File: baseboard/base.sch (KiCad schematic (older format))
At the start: 35 parts, among them J1 Conn_02x05_Odd_Even, J2 Barrel_Jack, J3 Barrel_Jack, J4 Conn_01x03_Male, Q1 BSS138, Q2 BSS138, Q3 BSS138, Q4 BSS138, Q5 BSS138, SW1 SW_Push, SW2 SW_Push, SW3 SW_Push, SW4 SW_Push, SW5 SW_Push, SW6 SW_Push, U1 WeMos_mini, U2 DS3231RTCModule, U3 NCH6100HVNixiePSU, U4 LM2596BuckConverterModule

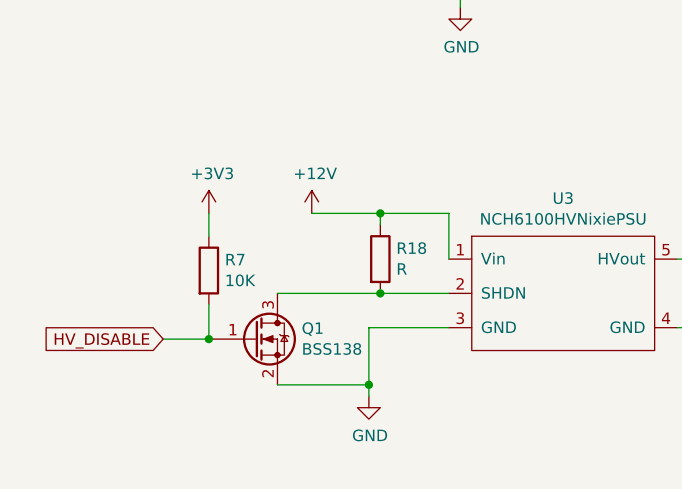
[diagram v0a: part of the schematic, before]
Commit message: Fix pulldown
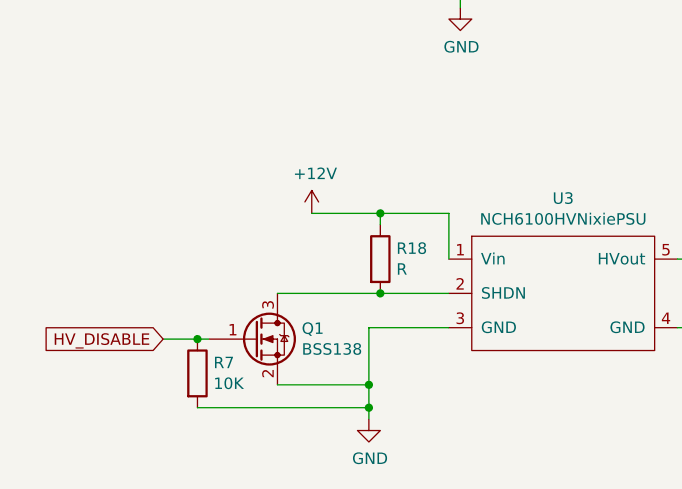
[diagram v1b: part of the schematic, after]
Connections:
- net +3V3: no longer R7.1
- net GND: now also R7.2
- net HV_DISABLE: now also R7.1; no longer R7.2
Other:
- moved on the sheet: R7
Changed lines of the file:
@@
 L power:GND #PWR0130
 U 1 1 5DC41A7F
-P 2050 6750
-F 0 "#PWR0130" H 2050 6500 50  0001 C CNN
-F 1 "GND" H 2055 6577 50  0000 C CNN
-F 2 "" H 2050 6750 50  0001 C CNN
-F 3 "" H 2050 6750 50  0001 C CNN
-	1    2050 6750
+P 2050 6850
+F 0 "#PWR0130" H 2050 6600 50  0001 C CNN
+F 1 "GND" H 2055 6677 50  0000 C CNN
+F 2 "" H 2050 6850 50  0001 C CNN
+F 3 "" H 2050 6850 50  0001 C CNN
+	1    2050 6850
 	1    0    0    -1
 $EndComp
@@
 	1650 6700 2050 6700
 Connection ~ 2050 6700
-Wire Wire Line
-	2050 6700 2050 6750
-Wire Wire Line
-	1150 6500 1350 6500
 $Comp
 L Transistor_FET:BSS138 Q5
@@
 Text GLabel 2550 1550 2    50   Input ~ 0
 SW_2
-$Comp
-L Device:R R7
-U 1 1 5DE5FC03
-P 1350 6200
-F 0 "R7" H 1420 6246 50  0000 L CNN
-F 1 "10K" H 1420 6155 50  0000 L CNN
-F 2 "Resistor_SMD:R_0805_2012Metric_Pad1.15x1.40mm_HandSolder" V 1280 6200 50  0001 C CNN
-F 3 "~" H 1350 6200 50  0001 C CNN
-	1    1350 6200
-	1    0    0    -1
-$EndComp
-$Comp
-L power:+3V3 #PWR0120
-U 1 1 5DE60E59
-P 1350 5950
-F 0 "#PWR0120" H 1350 5800 50  0001 C CNN
-F 1 "+3V3" H 1365 6123 50  0000 C CNN
-F 2 "" H 1350 5950 50  0001 C CNN
-F 3 "" H 1350 5950 50  0001 C CNN
-	1    1350 5950
-	1    0    0    -1
-$EndComp
+Wire Wire Line
+	2100 4700 3250 4700
+Wire Wire Line
+	2100 4550 3200 4550
 $Comp
 L Transistor_FET:BSS138 Q1
@@
 $EndComp
 Wire Wire Line
-	1350 6050 1350 5950
-Wire Wire Line
-	1350 6350 1350 6500
-Connection ~ 1350 6500
-Wire Wire Line
-	2100 4700 3250 4700
-Wire Wire Line
-	2100 4550 3200 4550
+	1150 6500 1300 6500
+$Comp
+L Device:R R7
+U 1 1 5DE5FC03
+P 1300 6650
+F 0 "R7" H 1370 6696 50  0000 L CNN
+F 1 "10K" H 1370 6605 50  0000 L CNN
+F 2 "Resistor_SMD:R_0805_2012Metric_Pad1.15x1.40mm_HandSolder" V 1230 6650 50  0001 C CNN
+F 3 "~" H 1300 6650 50  0001 C CNN
+	1    1300 6650
+	1    0    0    -1
+$EndComp
+Wire Wire Line
+	2050 6700 2050 6800
+Connection ~ 1300 6500
+Wire Wire Line
+	1300 6500 1350 6500
+Wire Wire Line
+	1300 6800 2050 6800
+Connection ~ 2050 6800
+Wire Wire Line
+	2050 6800 2050 6850
 $EndSCHEMATC
